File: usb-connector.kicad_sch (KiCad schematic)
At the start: 4 parts, among them J4 Pogo Pins, U3 USBLC6-2SC6

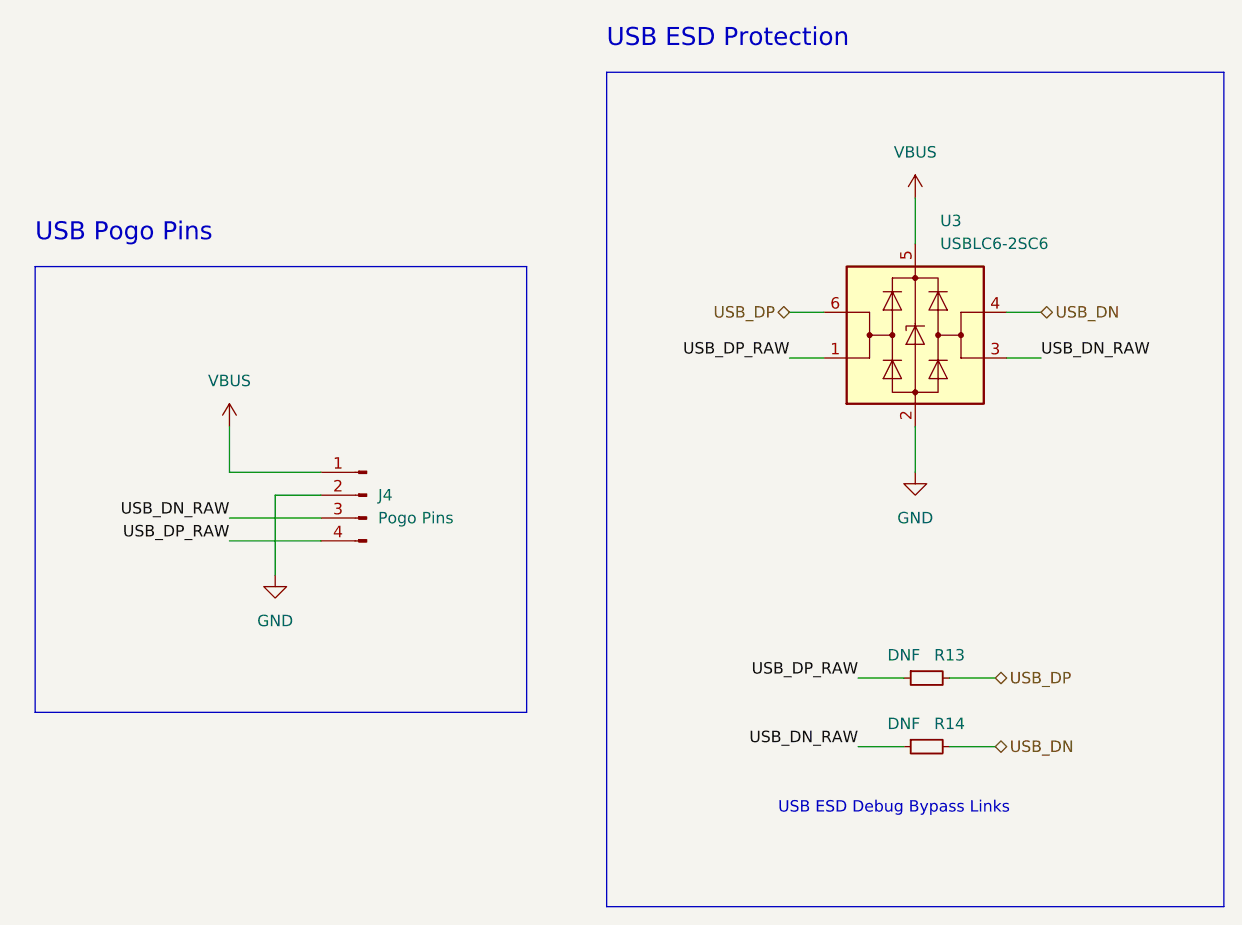
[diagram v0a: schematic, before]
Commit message: Add: Improved layout
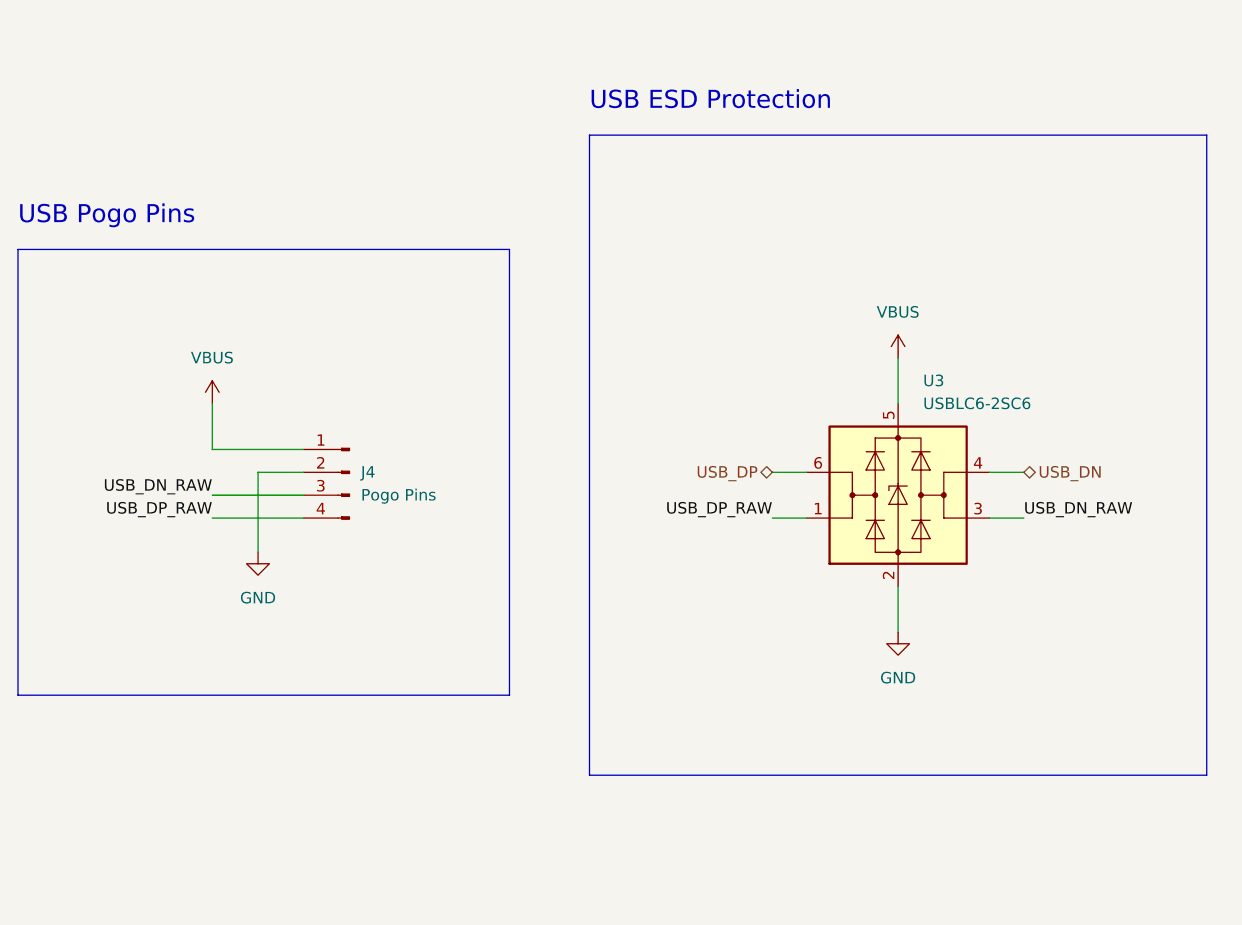
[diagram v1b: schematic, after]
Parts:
- removed R13, R14: DNF, Resistor_SMD:R_0402_1005Metric, symbol Device:R_Small
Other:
- note removed: "USB ESD Debug Bypass Links"
- moved on the sheet: J4, U3

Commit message: Change: Separate boards rather than using mousebites
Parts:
- J4: footprint Connector_PinHeader_2.00mm:PinHeader_1x04_P2.00mm_Vertical -> art:PogoPins; Int @ 10 (none) -> 2.13; MPN (none) -> 836-22-004-10-001101; Mfr (none) -> Mill-Max; SKU (none) -> 575-8362200410001101; Stock Situation (none) -> OK @ 2Nov2022; Vendor (none) -> Mouser
- U3: Int @ 10 (none) -> 0.554; MPN (none) -> USBLC6-2SC6; Mfr (none) -> STMicroelectronics; SKU (none) -> 511-USBLC6-2SC6; Stock Situation (none) -> OK @ 2Nov2022; Vendor (none) -> Mouser
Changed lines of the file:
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@@
+      (effects (font (size 1.27 1.27)) hide)
+    )
+    (property "Int @ 10" "0.554" (id 4) (at 183.515 102.87 0)
+      (effects (font (size 1.27 1.27)) hide)
+    )
+    (property "MPN" "USBLC6-2SC6" (id 5) (at 183.515 102.87 0)
+      (effects (font (size 1.27 1.27)) hide)
+    )
+    (property "Mfr" "STMicroelectronics" (id 6) (at 183.515 102.87 0)
+      (effects (font (size 1.27 1.27)) hide)
+    )
+    (property "SKU" "511-USBLC6-2SC6" (id 7) (at 183.515 102.87 0)
+      (effects (font (size 1.27 1.27)) hide)
+    )
+    (property "Stock Situation" "OK @ 2Nov2022" (id 8) (at 183.515 102.87 0)
+      (effects (font (size 1.27 1.27)) hide)
+    )
+    (property "Vendor" "Mouser" (id 9) (at 183.515 102.87 0)
       (effects (font (size 1.27 1.27)) hide)
     )
@@
       (effects (font (size 1.27 1.27)) (justify right))
     )
-    (property "Footprint" "Connector_PinHeader_2.00mm:PinHeader_1x04_P2.00mm_Vertical" (id 2) (at 122.555 100.33 0)
+    (property "Footprint" "art:PogoPins" (id 2) (at 122.555 100.33 0)
       (effects (font (size 1.27 1.27)) hide)
     )
@@
       (effects (font (size 1.27 1.27)) hide)
     )
+    (property "Int @ 10" "2.13" (id 4) (at 122.555 100.33 0)
+      (effects (font (size 1.27 1.27)) hide)
+    )
+    (property "MPN" "836-22-004-10-001101" (id 5) (at 122.555 100.33 0)
+      (effects (font (size 1.27 1.27)) hide)
+    )
+    (property "Mfr" "Mill-Max" (id 6) (at 122.555 100.33 0)
+      (effects (font (size 1.27 1.27)) hide)
+    )
+    (property "SKU" "575-8362200410001101" (id 7) (at 122.555 100.33 0)
+      (effects (font (size 1.27 1.27)) hide)
+    )
+    (property "Stock Situation" "OK @ 2Nov2022" (id 8) (at 122.555 100.33 0)
+      (effects (font (size 1.27 1.27)) hide)
+    )
+    (property "Vendor" "Mouser" (id 9) (at 122.555 100.33 0)
+      (effects (font (size 1.27 1.27)) hide)
+    )

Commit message: Add: Gerbers for Rev2
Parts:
- J4: Int @ 10 2.13 -> 0.75; Mfr Mill-Max -> RTLecs; SKU 575-8362200410001101 -> 4000689589714; Vendor Mouser -> AliExpress
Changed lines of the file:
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@@
       (effects (font (size 1.27 1.27)) hide)
     )
-    (property "Int @ 10" "2.13" (id 4) (at 122.555 100.33 0)
+    (property "Int @ 10" "0.75" (id 4) (at 122.555 100.33 0)
       (effects (font (size 1.27 1.27)) hide)
     )
@@
       (effects (font (size 1.27 1.27)) hide)
     )
-    (property "Mfr" "Mill-Max" (id 6) (at 122.555 100.33 0)
+    (property "Mfr" "RTLecs" (id 6) (at 122.555 100.33 0)
       (effects (font (size 1.27 1.27)) hide)
     )
-    (property "SKU" "575-8362200410001101" (id 7) (at 122.555 100.33 0)
+    (property "SKU" "4000689589714" (id 7) (at 122.555 100.33 0)
       (effects (font (size 1.27 1.27)) hide)
     )
@@
       (effects (font (size 1.27 1.27)) hide)
     )
-    (property "Vendor" "Mouser" (id 9) (at 122.555 100.33 0)
+    (property "Vendor" "AliExpress" (id 9) (at 122.555 100.33 0)
       (effects (font (size 1.27 1.27)) hide)
     )
